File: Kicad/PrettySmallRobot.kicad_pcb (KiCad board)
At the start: 2 copper layers, 16.7 x 25 mm, 55 parts, among them J1 TYPE-C-31-M-12, J2 MOTORA_1, J3 MOTORA_2, J4 MOTORB_1, J5 MOTORB_2, J6 BATT+, J7 GND, SW1 SW_Push, SW2 SW_Push, U1 DRV8837, U2 DRV8837, U3 MCP73831-2ACI_MC, U4 ESP32-S2, U6 AP2112K-3.3, Y1 12pF/40MHz

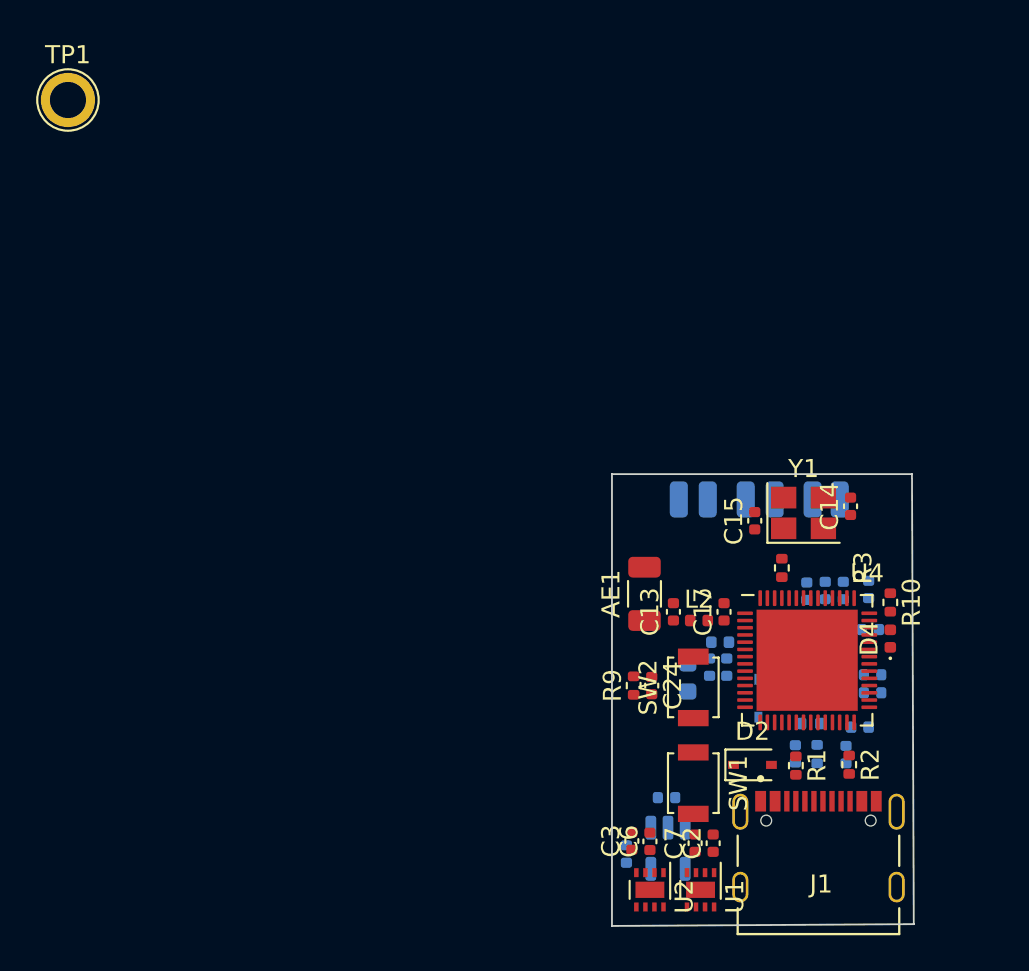
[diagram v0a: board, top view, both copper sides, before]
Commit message: routing bout 70% done
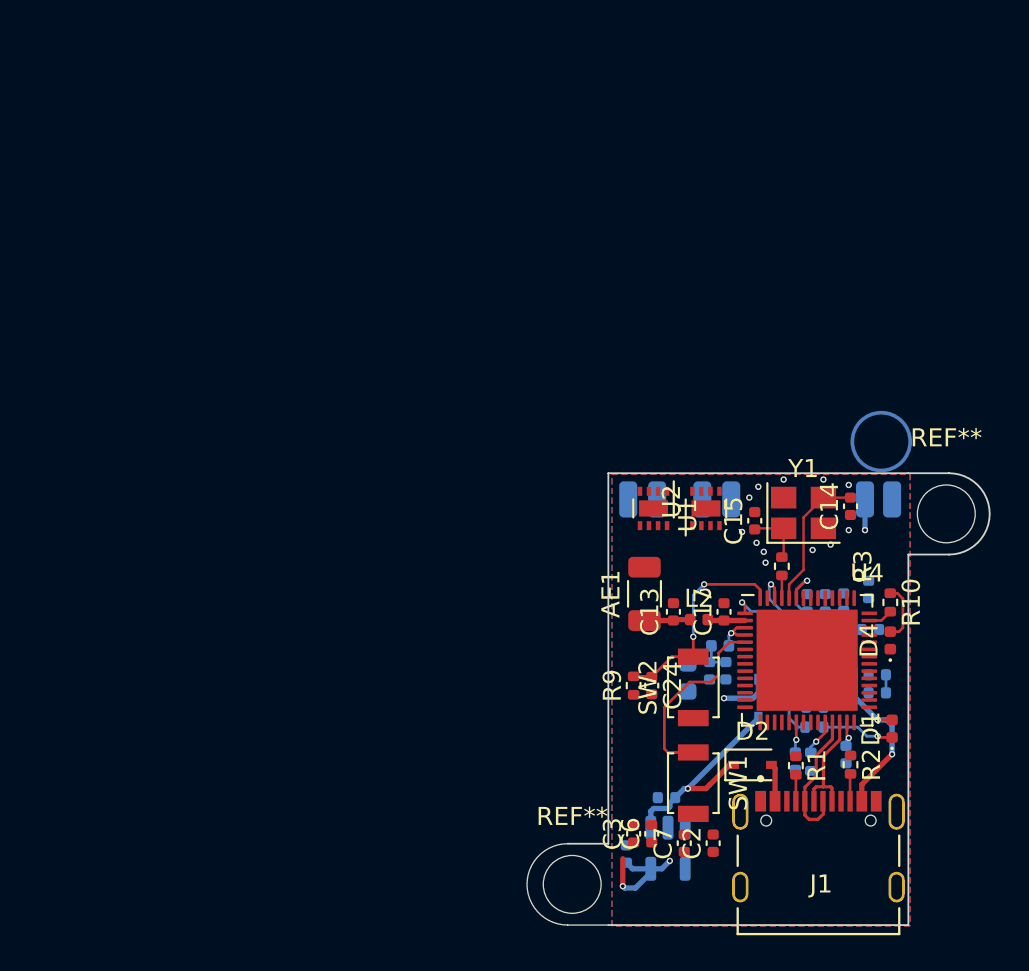
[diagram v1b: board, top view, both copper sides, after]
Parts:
- removed TP1: TEST, TestPoint:TestPoint_Plated_Hole_D2.0mm
- added REF**: MountingHole_3.2mm_M3, MountingHole:MountingHole_3.2mm_M3, F.Cu at (146.0, 98.7)
- added REF**: MountingHole_3.2mm_M3_ISO14580, MountingHole:MountingHole_3.2mm_M3_ISO14580, F.Cu at (125.3, 119.2)
- D1: moved to F.Cu
- moved U2 21.3 mm to (132.7, 98.4), turned to 90 degrees
- moved U1 21.3 mm to (129.8, 98.4)
- moved C21 4.50 mm to (138.7, 109.4)
- moved J6 2.90 mm to (141.5, 97.9)
- moved J7 2.90 mm to (143.0, 97.9)
- moved J2 2.80 mm to (130.0, 97.9)
- moved J5 2.80 mm to (128.4, 97.9)
- moved J3 2.40 mm to (134.1, 97.9)
- moved J4 2.40 mm to (132.5, 97.9)
- moved C19 2.13 mm to (140.3, 103.6), turned to 90 degrees
- moved C20 2.11 mm to (138.3, 103.6), turned to 90 degrees
- moved D1 1.79 mm to (143.0, 110.6), turned to 90 degrees
- moved R6 1.08 mm to (138.7, 105.7)
- moved C18 0.68 mm to (139.3, 103.6), turned to 90 degrees
- moved C7 0.60 mm to (131.5, 116.9)
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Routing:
- net +BATT: track 0.00 -> 20.2 mm, vias 0 -> 2
- net /VDDA: track 0.00 -> 14.2 mm, vias 0 -> 3
- net /VBUS: track 0.00 -> 13.6 mm, vias 0 -> 2
- net +3V3: track 0.00 -> 12.9 mm, vias 0 -> 4
- net Net-(C22-Pad1): track 0.00 -> 12.2 mm, vias 0 -> 1
- net /~{RESET}: track 0.00 -> 11.7 mm, vias 0 -> 2
- net /BOOT: track 0.00 -> 10.6 mm
- net Net-(U4-Pad52): track 0.00 -> 7.85 mm
- net /D-: track 0.00 -> 7.72 mm
- net /D+: track 0.00 -> 6.42 mm
- net Net-(D1-Pad1): track 0.00 -> 4.03 mm, vias 0 -> 1
- net Net-(R3-Pad1): track 0.00 -> 3.26 mm
- net Net-(D4-Pad2): track 0.00 -> 3.22 mm
- net Net-(R5-Pad2): track 0.00 -> 2.77 mm
- net Net-(AE1-Pad1): track 0.00 -> 2.55 mm
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- added copper zone on In2.Cu, net +3V3
- added copper zone on B.Cu, net GND
- added copper zone on F.Cu, net GND
- added copper zone on In1.Cu, net GND
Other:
- board size 16.7 x 25 mm -> 25.6 x 25 mm
- copper layers 2 -> 4
